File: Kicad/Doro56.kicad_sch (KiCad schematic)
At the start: 75 parts, among them J1 MJ-4PP-9, SW1 SW_Push_45deg, SW10 SW_Push_45deg, SW11 SW_Push_45deg, SW12 SW_Push_45deg, SW13 SW_Push_45deg, SW14 SW_Push_45deg, SW15 SW_Push_45deg, SW16 SW_Push_45deg, SW17 SW_Push_45deg, SW18 SW_Push_45deg, SW19 SW_Push_45deg, SW2 SW_Push_45deg, SW20 SW_Push_45deg, SW21 SW_Push_45deg, SW22 SW_Push_45deg, SW23 SW_Push_45deg, SW24 SW_Push_45deg, SW25 SW_Push_45deg, SW26 SW_Push_45deg, SW27 SW_Push_45deg, SW28 SW_Push_45deg, SW29 SW_Push_45deg, SW3 SW_Push_45deg, SW30 SW_Push_45deg, SW31 SW_Push_45deg, SW33 RotaryEncoder_Switch, SW34 SW_SPDT, SW4 SW_Push_45deg, SW5 SW_Push_45deg, SW6 SW_Push_45deg, SW7 SW_Push_45deg, SW8 SW_Push_45deg, SW9 SW_Push_45deg, U1 ProMicro

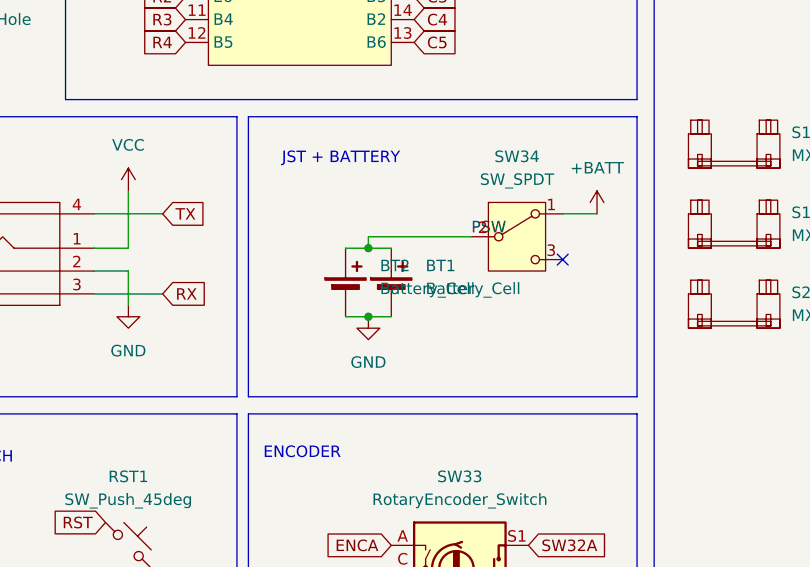
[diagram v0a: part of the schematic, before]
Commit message: 1.2
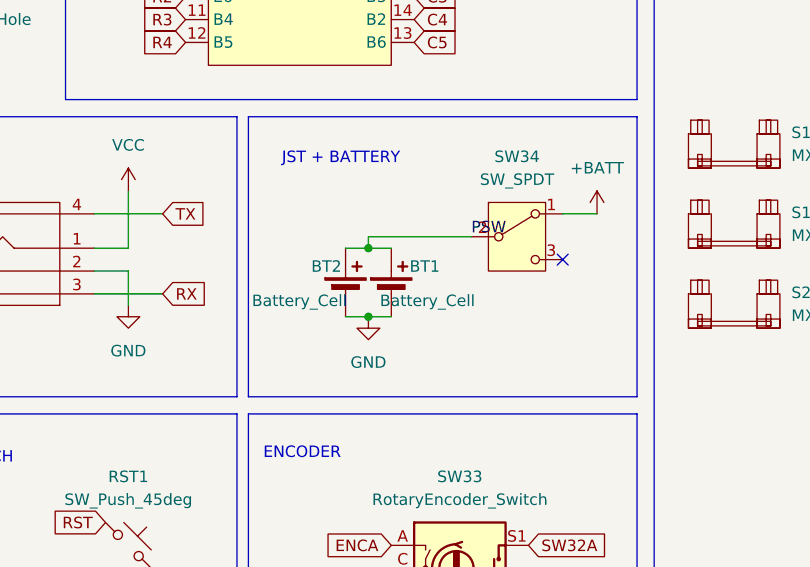
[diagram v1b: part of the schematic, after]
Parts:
- BT1: footprint GHN:JST_PH_reversible_vert -> GHN:JST_PH_2P_Reversible
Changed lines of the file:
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@@
 		(dnp no)
 		(property "Reference" "BT2"
-			(at 96.52 83.2484 0)
+			(at 88.9 83.312 0)
 			(effects
 				(font
@@
 		)
 		(property "Value" "Battery_Cell"
-			(at 96.52 85.7884 0)
+			(at 82.296 87.122 0)
 			(effects
 				(font
@@
 		(dnp no)
 		(property "Reference" "BT1"
-			(at 101.6 83.2484 0)
+			(at 99.822 83.312 0)
 			(effects
 				(font
@@
 		)
 		(property "Value" "Battery_Cell"
-			(at 101.6 85.7884 0)
+			(at 96.52 87.122 0)
 			(effects
 				(font
@@
 			)
 		)
-		(property "Footprint" "GHN:JST_PH_reversible_vert"
+		(property "Footprint" "GHN:JST_PH_2P_Reversible"
 			(at 97.79 84.836 90)
 			(effects
